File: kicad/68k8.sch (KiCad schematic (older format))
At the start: 45 parts

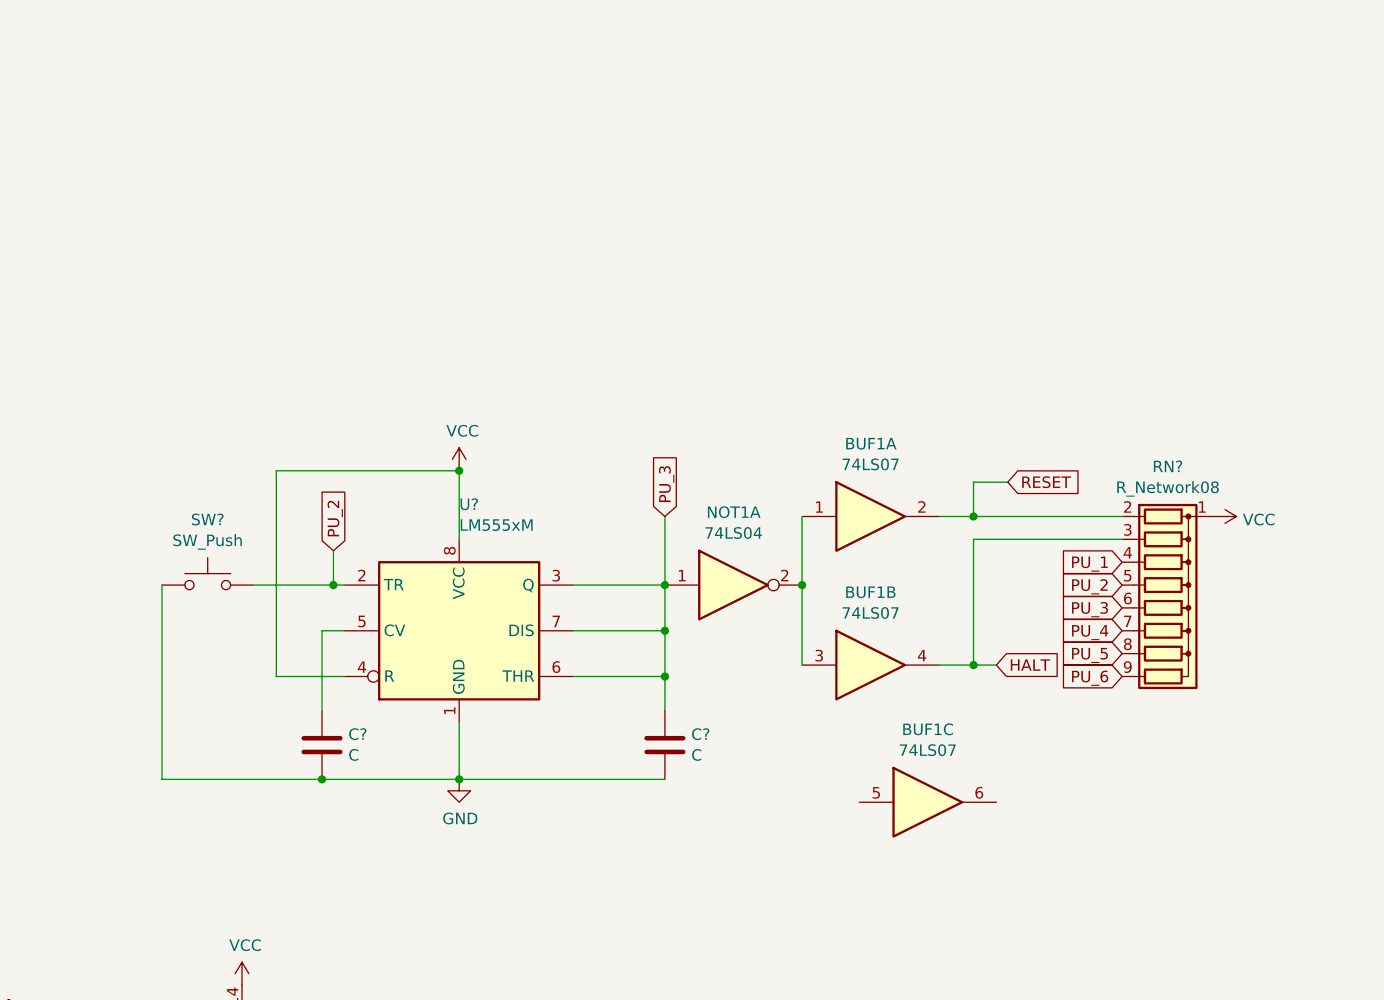
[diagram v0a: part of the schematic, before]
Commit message: updates from a long time ago
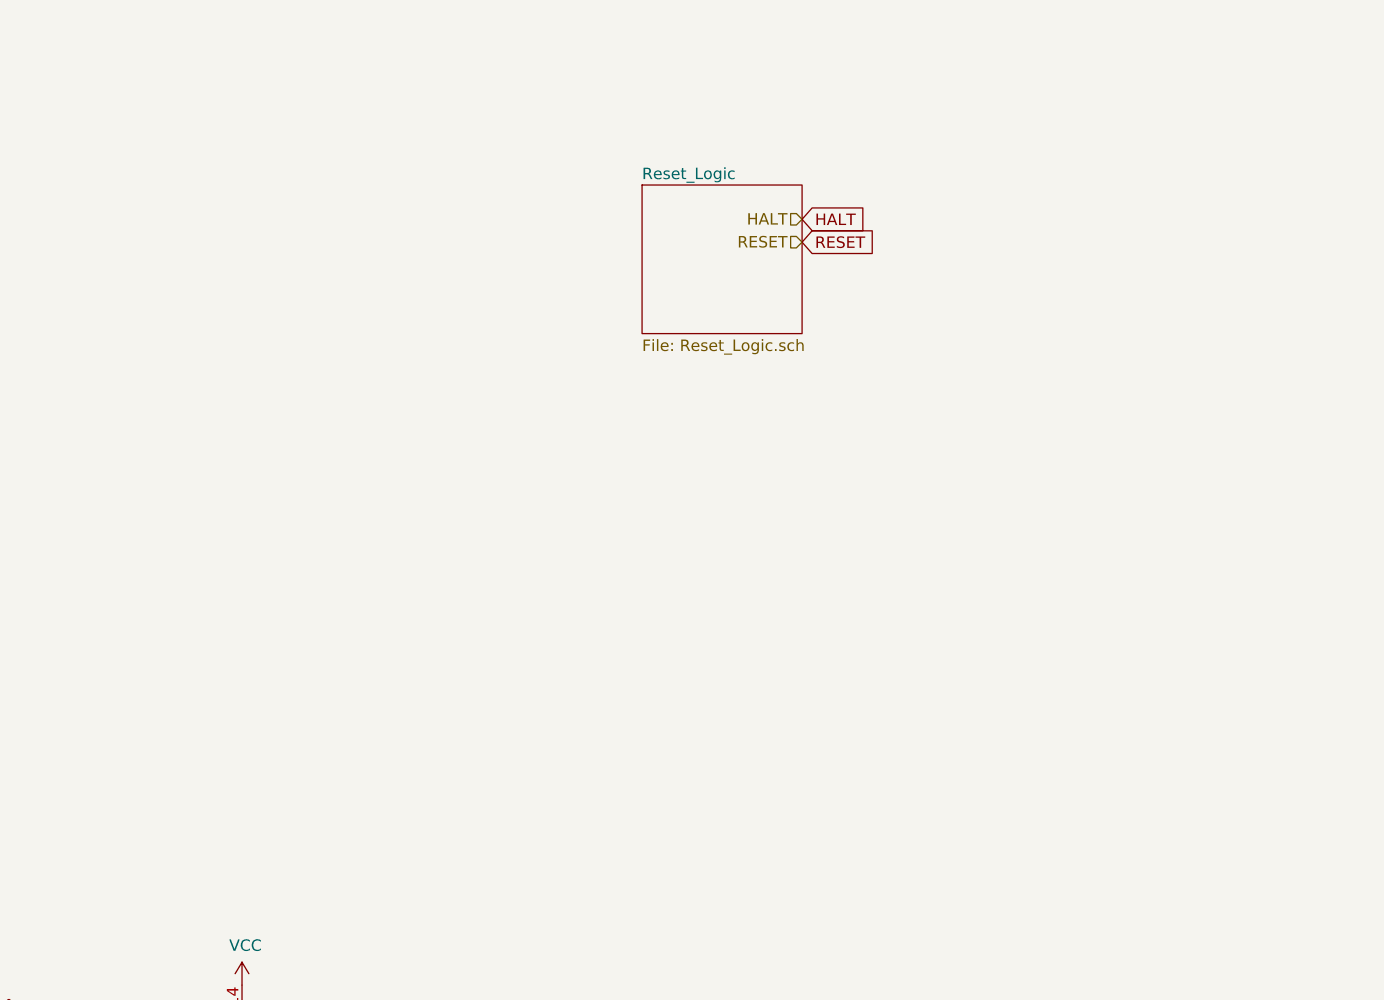
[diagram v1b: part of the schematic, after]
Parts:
- removed BUF1: 74LS07, symbol 74xx:74LS07
- removed C? (x2): C, symbol Device:C
- removed unit 1 of NOT1
- removed RN?: R_Network08, Resistor_THT:R_Array_SIP9, symbol Device:R_Network08
- removed SW?: SW_Push, symbol Switch:SW_Push
- removed U?: LM555xM, Package_SO:SOIC-8_3.9x4.9mm_P1.27mm, symbol Timer:LM555xM
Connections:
- net labels removed: PU_2, PU_3, PU_6
- wire segments 245 -> 214
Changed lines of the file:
@@
 $Descr A2 23386 16535
 encoding utf-8
-Sheet 1 2
+Sheet 1 3
 Title "68k8 SBC"
 Date "2021-07-16"
@@
 Text Label 3600 10650 0    50   ~ 0
 A3
-$Comp
-L 74xx:74LS07 BUF1
-U 1 1 614D70EA
-P 20200 12950
-F 0 "BUF1" H 20200 13267 50  0000 C CNN
-F 1 "74LS07" H 20200 13176 50  0000 C CNN
-F 2 "" H 20200 12950 50  0001 C CNN
-F 3 "www.ti.com/lit/ds/symlink/sn74ls07.pdf" H 20200 12950 50  0001 C CNN
-	1    20200 12950
-	1    0    0    -1
-$EndComp
-$Comp
-L 74xx:74LS07 BUF1
-U 2 1 614D7E5F
-P 20200 13600
-F 0 "BUF1" H 20200 13917 50  0000 C CNN
-F 1 "74LS07" H 20200 13826 50  0000 C CNN
-F 2 "" H 20200 13600 50  0001 C CNN
-F 3 "www.ti.com/lit/ds/symlink/sn74ls07.pdf" H 20200 13600 50  0001 C CNN
-	2    20200 13600
-	1    0    0    -1
-$EndComp
-$Comp
-L 74xx:74LS07 BUF1
-U 3 1 614D93B5
-P 20450 14200
-F 0 "BUF1" H 20450 14517 50  0000 C CNN
-F 1 "74LS07" H 20450 14426 50  0000 C CNN
-F 2 "" H 20450 14200 50  0001 C CNN
-F 3 "www.ti.com/lit/ds/symlink/sn74ls07.pdf" H 20450 14200 50  0001 C CNN
-	3    20450 14200
-	1    0    0    -1
-$EndComp
-Wire Wire Line
-	20500 12950 20650 12950
-Wire Wire Line
-	20500 13600 20650 13600
-Wire Wire Line
-	20650 12950 20650 12800
-Wire Wire Line
-	20650 12800 20800 12800
-Text GLabel 20800 12800 2    50   Input ~ 0
-RESET
-Text GLabel 20750 13600 2    50   Input ~ 0
-HALT
-Wire Wire Line
-	20650 13600 20750 13600
-Connection ~ 20650 13600
-$Comp
-L Timer:LM555xM U?
-U 1 1 61569D76
-P 18400 13450
-F 0 "U?" H 18400 14031 50  0000 L TNN
-F 1 "LM555xM" H 18400 13940 50  0000 L TNN
-F 2 "Package_SO:SOIC-8_3.9x4.9mm_P1.27mm" H 19250 13050 50  0001 C CNN
-F 3 "http://www.ti.com/lit/ds/symlink/lm555.pdf" H 19250 13050 50  0001 C CNN
-	1    18400 13450
-	1    0    0    -1
-$EndComp
-$Comp
-L power:GND #PWR?
-U 1 1 6156DCD9
-P 18400 14100
-F 0 "#PWR?" H 18400 13850 50  0001 C CNN
-F 1 "GND" H 18405 13927 50  0000 C CNN
-F 2 "" H 18400 14100 50  0001 C CNN
-F 3 "" H 18400 14100 50  0001 C CNN
-	1    18400 14100
-	1    0    0    -1
-$EndComp
-$Comp
-L Switch:SW_Push SW?
-U 1 1 6156FADE
-P 17300 13250
-F 0 "SW?" H 17300 13535 50  0000 C CNN
-F 1 "SW_Push" H 17300 13444 50  0000 C CNN
-F 2 "" H 17300 13450 50  0001 C CNN
-F 3 "~" H 17300 13450 50  0001 C CNN
-	1    17300 13250
-	1    0    0    -1
-$EndComp
-$Comp
-L power:VCC #PWR?
-U 1 1 6156CD1A
-P 18400 12750
-F 0 "#PWR?" H 18400 12600 50  0001 C CNN
-F 1 "VCC" H 18415 12923 50  0000 C CNN
-F 2 "" H 18400 12750 50  0001 C CNN
-F 3 "" H 18400 12750 50  0001 C CNN
-	1    18400 12750
-	1    0    0    -1
-$EndComp
-$Comp
-L Device:C C?
-U 1 1 61618BC8
-P 17800 13950
-F 0 "C?" H 17915 13996 50  0000 L CNN
-F 1 "C" H 17915 13905 50  0000 L CNN
-F 2 "" H 17838 13800 50  0001 C CNN
-F 3 "~" H 17800 13950 50  0001 C CNN
-	1    17800 13950
-	1    0    0    -1
-$EndComp
-Wire Wire Line
-	18400 13850 18400 14100
-Wire Wire Line
-	17100 14100 17100 13250
-Connection ~ 18400 14100
-Wire Wire Line
-	18900 13250 19300 13250
-Wire Wire Line
-	19300 13250 19300 12950
-Wire Wire Line
-	18900 13450 19300 13450
-Wire Wire Line
-	19300 13450 19300 13250
-Connection ~ 19300 13250
-Wire Wire Line
-	18900 13650 19300 13650
-Wire Wire Line
-	19300 13650 19300 13450
-Connection ~ 19300 13450
-$Comp
-L Device:C C?
-U 1 1 616C0EA1
-P 19300 13950
-F 0 "C?" H 19415 13996 50  0000 L CNN
-F 1 "C" H 19415 13905 50  0000 L CNN
-F 2 "" H 19338 13800 50  0001 C CNN
-F 3 "~" H 19300 13950 50  0001 C CNN
-	1    19300 13950
-	1    0    0    -1
-$EndComp
-Wire Wire Line
-	18400 14100 19300 14100
 Text GLabel 1100 4100 0    50   Input ~ 0
 HALT
@@
 Text GLabel 3750 11150 0    50   Input ~ 0
 RESET
-$Comp
-L 74xx:74LS04 NOT1
-U 1 1 6101E3F3
-P 19600 13250
-F 0 "NOT1" H 19600 13567 50  0000 C CNN
-F 1 "74LS04" H 19600 13476 50  0000 C CNN
-F 2 "" H 19600 13250 50  0001 C CNN
-F 3 "http://www.ti.com/lit/gpn/sn74LS04" H 19600 13250 50  0001 C CNN
-	1    19600 13250
-	1    0    0    -1
-$EndComp
 $Comp
 L 74xx:74LS04 NOT1
@@
 	1    0    0    -1
 $EndComp
-Connection ~ 19300 13650
-Wire Wire Line
-	19300 13650 19300 13800
-Wire Wire Line
-	19900 12950 19900 13250
-Connection ~ 19900 13250
-Wire Wire Line
-	19900 13250 19900 13600
-Connection ~ 17800 14100
-Wire Wire Line
-	17100 14100 17800 14100
-Wire Wire Line
-	17900 13450 17800 13450
-Wire Wire Line
-	17800 13450 17800 13800
-Wire Wire Line
-	17900 13650 17600 13650
-Wire Wire Line
-	17800 14100 18400 14100
-Wire Wire Line
-	20650 13600 20650 13050
-$Comp
-L power:VCC #PWR?
-U 1 1 61522293
-P 21700 12950
-F 0 "#PWR?" H 21700 12800 50  0001 C CNN
-F 1 "VCC" V 21715 13078 50  0000 L CNN
-F 2 "" H 21700 12950 50  0001 C CNN
-F 3 "" H 21700 12950 50  0001 C CNN
-	1    21700 12950
-	0    1    1    0
-$EndComp
-Connection ~ 20650 12950
 $Comp
 L Interface_USB:MCP2221AxP U?
@@
 Wire Wire Line
 	7500 8450 8000 8450
-Text GLabel 21300 13150 0    50   Input ~ 0
-PU_1
 Text GLabel 7900 9550 2    50   Input ~ 0
 PU_1
-Text GLabel 21300 13250 0    50   Input ~ 0
-PU_2
-Text GLabel 21300 13350 0    50   Input ~ 0
-PU_3
-Text GLabel 17850 13100 1    50   Input ~ 0
-PU_2
-Text GLabel 19300 12950 1    50   Input ~ 0
-PU_3
-Wire Wire Line
-	17600 12750 18400 12750
 Wire Wire Line
 	19850 4650 19950 4650
@@
 Text GLabel 10550 11700 2    50   Input ~ 0
 RESET
-$Comp
-L Device:R_Network08 RN?
-U 1 1 61C4E53B
-P 21500 13350
-F 0 "RN?" V 20883 13350 50  0000 C CNN
-F 1 "R_Network08" V 20974 13350 50  0000 C CNN
-F 2 "Resistor_THT:R_Array_SIP9" V 21975 13350 50  0001 C CNN
-F 3 "http://www.vishay.com/docs/31509/csc.pdf" H 21500 13350 50  0001 C CNN
-	1    21500 13350
-	0    1    1    0
-$EndComp
-Wire Wire Line
-	20650 13050 21300 13050
-Wire Wire Line
-	20650 12950 21300 12950
-Text GLabel 21300 13450 0    50   Input ~ 0
-PU_4
-Text GLabel 21300 13550 0    50   Input ~ 0
-PU_5
-Text GLabel 21300 13650 0    50   Input ~ 0
-PU_6
 Text GLabel 900  2000 0    50   Input ~ 0
 MFP_IRQ
@@
 	-1   0    0    1
 $EndComp
-Wire Wire Line
-	17500 13250 17850 13250
-Wire Wire Line
-	17850 13250 17850 13100
-Connection ~ 17850 13250
-Wire Wire Line
-	17850 13250 17900 13250
-Wire Wire Line
-	17600 13650 17600 12750
-Wire Wire Line
-	18400 12750 18400 13050
-Connection ~ 18400 12750
 $Comp
 L 74xx:74LS21 4AND
@@
 Wire Wire Line
 	4950 15700 5350 15700
-Wire Bus Line
-	18100 4700 18100 5000
-Wire Bus Line
-	17400 900  17400 1300
-Wire Bus Line
-	3450 10250 3450 10650
-Wire Bus Line
-	9150 9300 9150 9800
-Wire Bus Line
-	4900 1600 4900 5000
-Wire Bus Line
-	7100 1600 7100 5000
-Wire Bus Line
-	9300 1600 9300 5000
-Wire Bus Line
-	3450 9350 3450 10150
-Wire Bus Line
-	3150 3900 3150 5000
-Wire Bus Line
-	10850 9400 10850 10200
-Wire Bus Line
-	3550 900  3550 2800
-Wire Bus Line
-	7400 900  7400 3200
-Wire Bus Line
-	5200 900  5200 3200
-Wire Bus Line
-	3200 900  3200 3500
 Connection ~ 5350 15700
 Wire Wire Line
@@
 $EndComp
 Connection ~ 4950 15700
+$Sheet
+S 19200 11500 700  650
+U 6110C011
+F0 "Reset_Logic" 50
+F1 "Reset_Logic.sch" 50
+$EndSheet
+Text HLabel 19900 11650 0    50   Input ~ 0
+HALT
+Text HLabel 19900 11750 0    50   Input ~ 0
+RESET
+Text GLabel 19900 11750 2    50   Input ~ 0
+RESET
+Text GLabel 19900 11650 2    50   Input ~ 0
+HALT
+Wire Bus Line
+	18100 4700 18100 5000
+Wire Bus Line
+	17400 900  17400 1300
+Wire Bus Line
+	3450 10250 3450 10650
+Wire Bus Line
+	9150 9300 9150 9800
+Wire Bus Line
+	4900 1600 4900 5000
+Wire Bus Line
+	7100 1600 7100 5000
+Wire Bus Line
+	9300 1600 9300 5000
+Wire Bus Line
+	3450 9350 3450 10150
+Wire Bus Line
+	3150 3900 3150 5000
+Wire Bus Line
+	10850 9400 10850 10200
+Wire Bus Line
+	3550 900  3550 2800
+Wire Bus Line
+	7400 900  7400 3200
+Wire Bus Line
+	5200 900  5200 3200
+Wire Bus Line
+	3200 900  3200 3500
 $EndSCHEMATC
